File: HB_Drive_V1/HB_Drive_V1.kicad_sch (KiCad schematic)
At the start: 0 parts

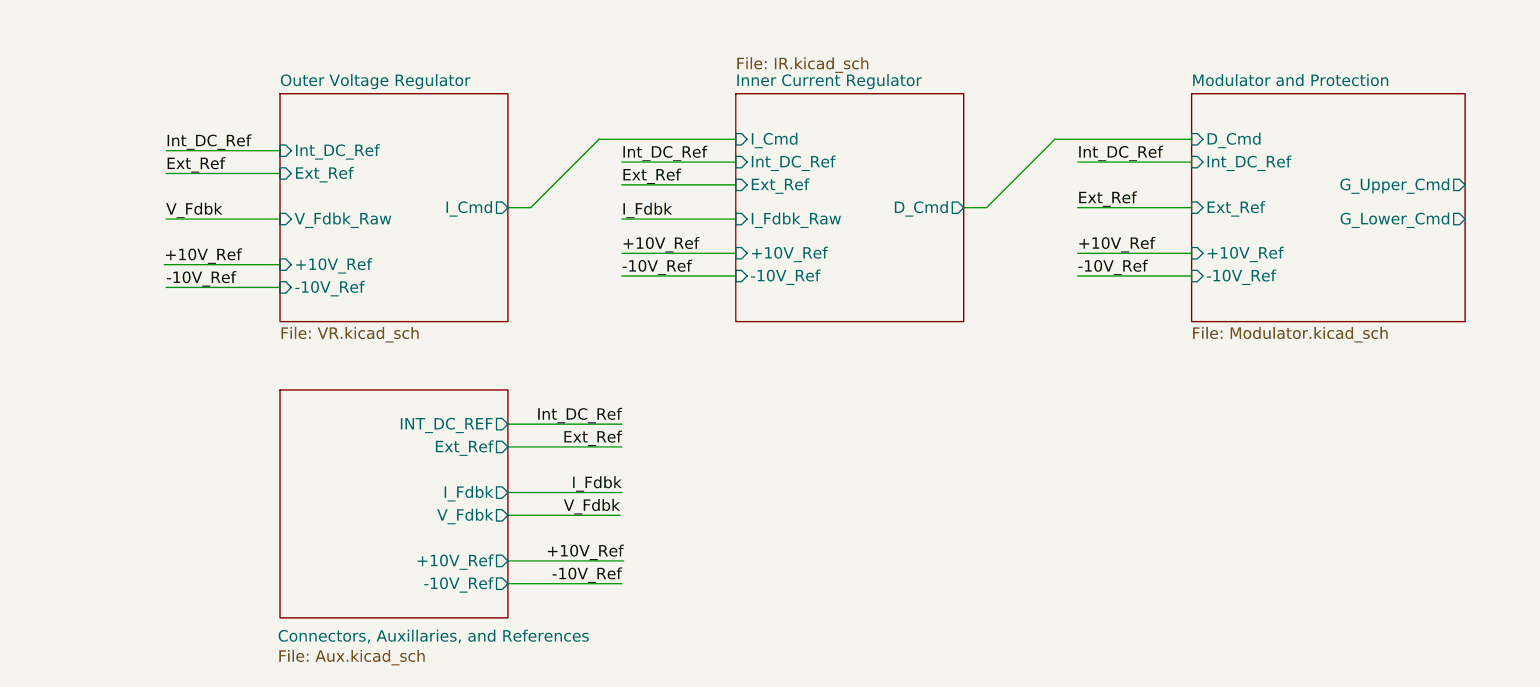
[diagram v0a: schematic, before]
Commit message: updates board to highest working copy
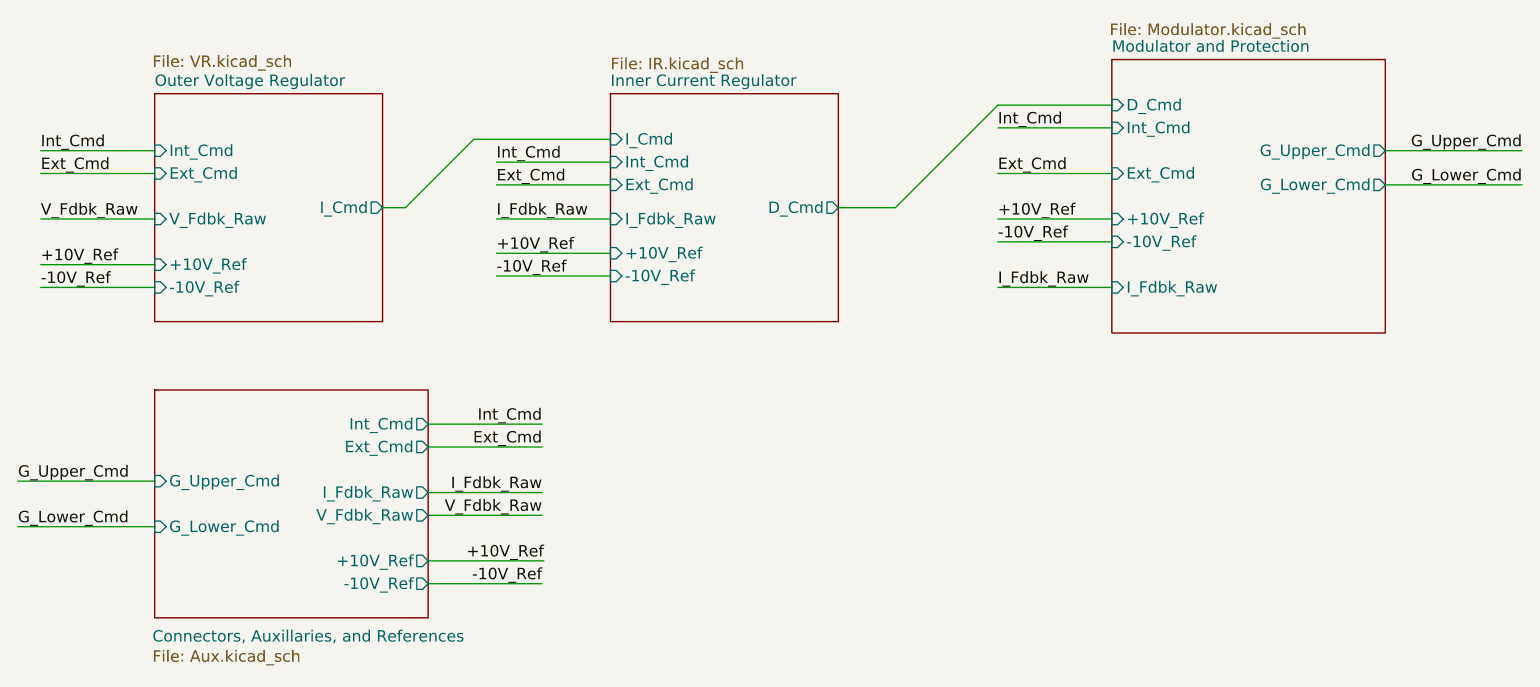
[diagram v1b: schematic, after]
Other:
- sheet Connectors, Auxillaries, and References ports: added Ext_Cmd, G_Lower_Cmd, G_Upper_Cmd, I_Fdbk_Raw, Int_Cmd, V_Fdbk_Raw; removed Ext_Ref, INT_DC_REF, I_Fdbk, V_Fdbk
- sheet Inner Current Regulator ports: added Ext_Cmd, Int_Cmd; removed Ext_Ref, Int_DC_Ref
- sheet Modulator and Protection ports: added Ext_Cmd, I_Fdbk_Raw, Int_Cmd; removed Ext_Ref, Int_DC_Ref
- sheet Outer Voltage Regulator ports: added Ext_Cmd, Int_Cmd; removed Ext_Ref, Int_DC_Ref
